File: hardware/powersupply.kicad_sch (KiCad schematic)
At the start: 15 parts, among them U1 h0536, U2 LD1117S33TR_SOT223

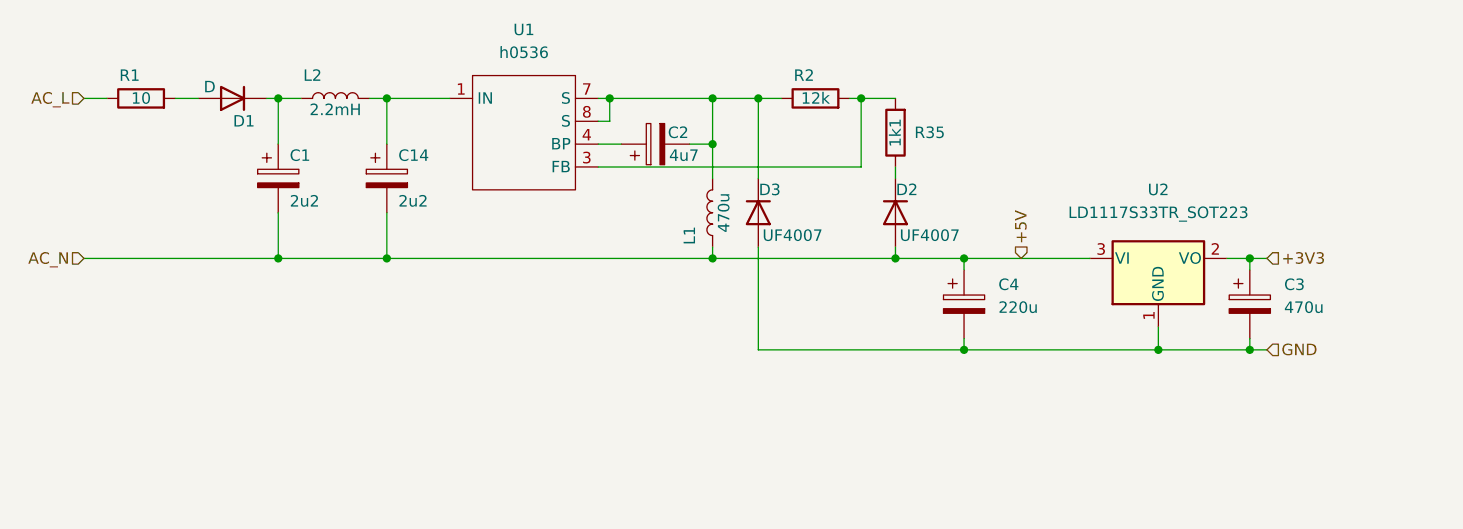
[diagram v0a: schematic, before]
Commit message: done routing
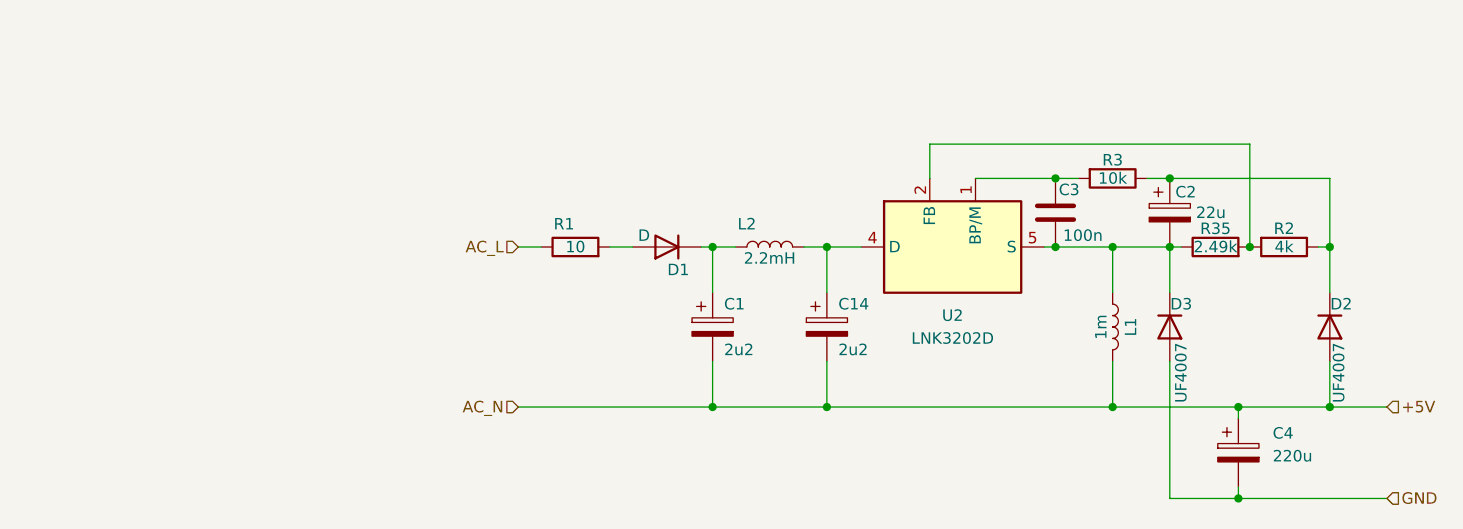
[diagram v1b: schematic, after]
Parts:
- removed C3: 470u, Capacitor_THT:CP_Radial_D8.0mm_P3.50mm, symbol Device:C_Polarized
- removed U1: h0536, Package_DIP:DIP-8_W7.62mm, symbol buck:h0536
- removed U2: LD1117S33TR_SOT223, Package_TO_SOT_SMD:SOT-223-3_TabPin2, symbol Regulator_Linear:LD1117S33TR_SOT223
- added C3: 100n, Capacitor_SMD:C_0603_1608Metric, symbol Device:C
- added R3: 10k, Resistor_SMD:R_0603_1608Metric, symbol Device:R
- added U2: LNK3202D, Package_SO:PowerIntegrations_SO-8C, symbol Regulator_Switching:LNK3202D
- C2: value 4u7 -> 22u
- L1: value 470u -> 1m
- R2: value 12k -> 4k
- R35: value 1k1 -> 2.49k
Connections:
- net +5V: now also L1.2; no longer L1.1
- net at D2.1 (K): now also C2.1, R2.1, R3.1; no longer R35.1
- net at R2.2, R35.2: now also U2.2 (FB)
- net at C2.2, D3.1 (K): now also L1.1, R35.1, C3.1, U2.5 (S), U2.6 (S), U2.7 (S), U2.8 (S); no longer L1.2, R2.1
- net at C14.1, L2.2: now also U2.4 (D)
- new net: C3.2, R3.2, U2.1 (BP/M)
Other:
- moved on the sheet: C1, C14, C2, C4, D1, D2, D3, L1, L2, R1, R2, R35
